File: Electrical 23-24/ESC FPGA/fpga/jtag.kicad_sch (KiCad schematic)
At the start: 0 parts

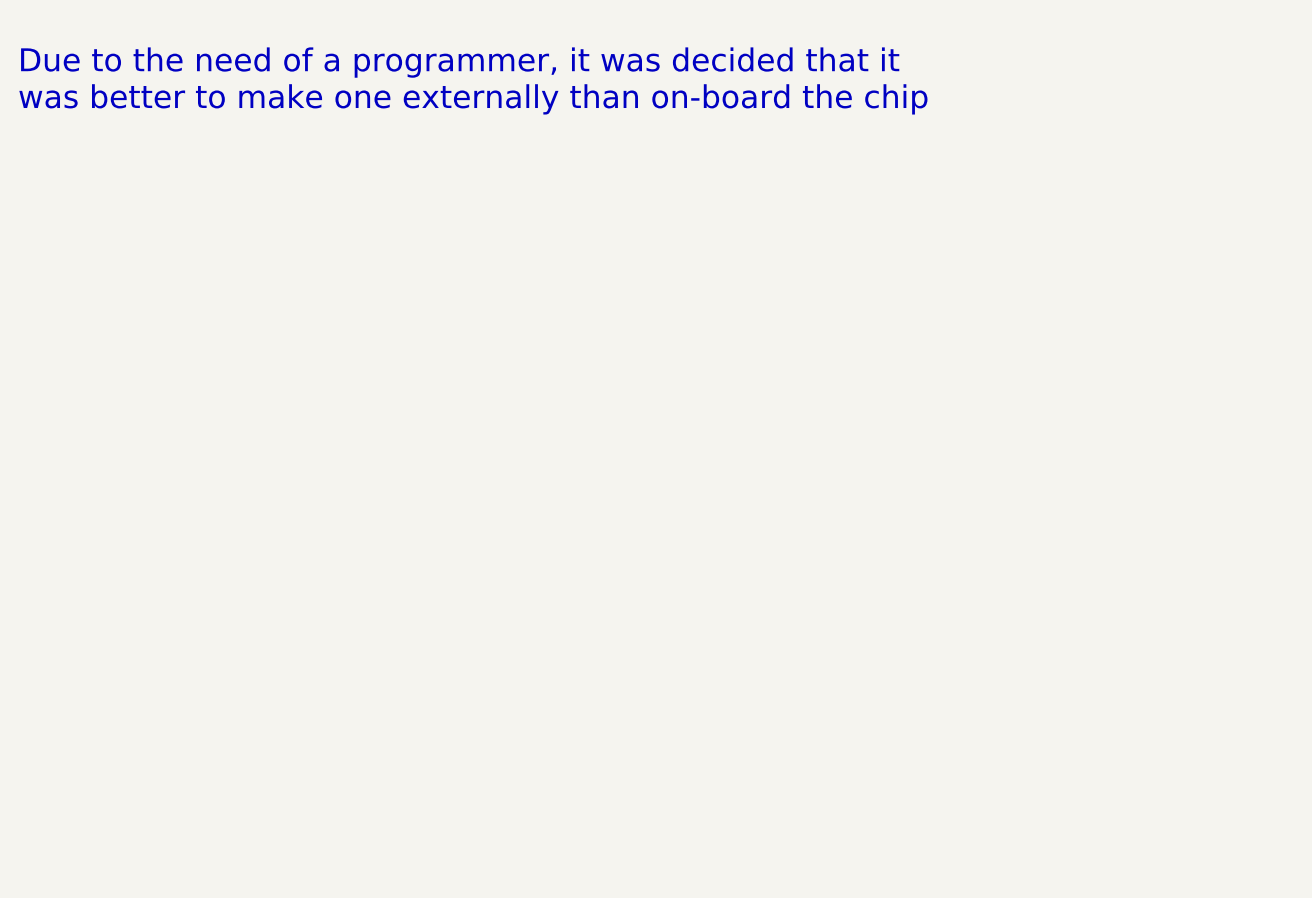
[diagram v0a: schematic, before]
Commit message: idk but something
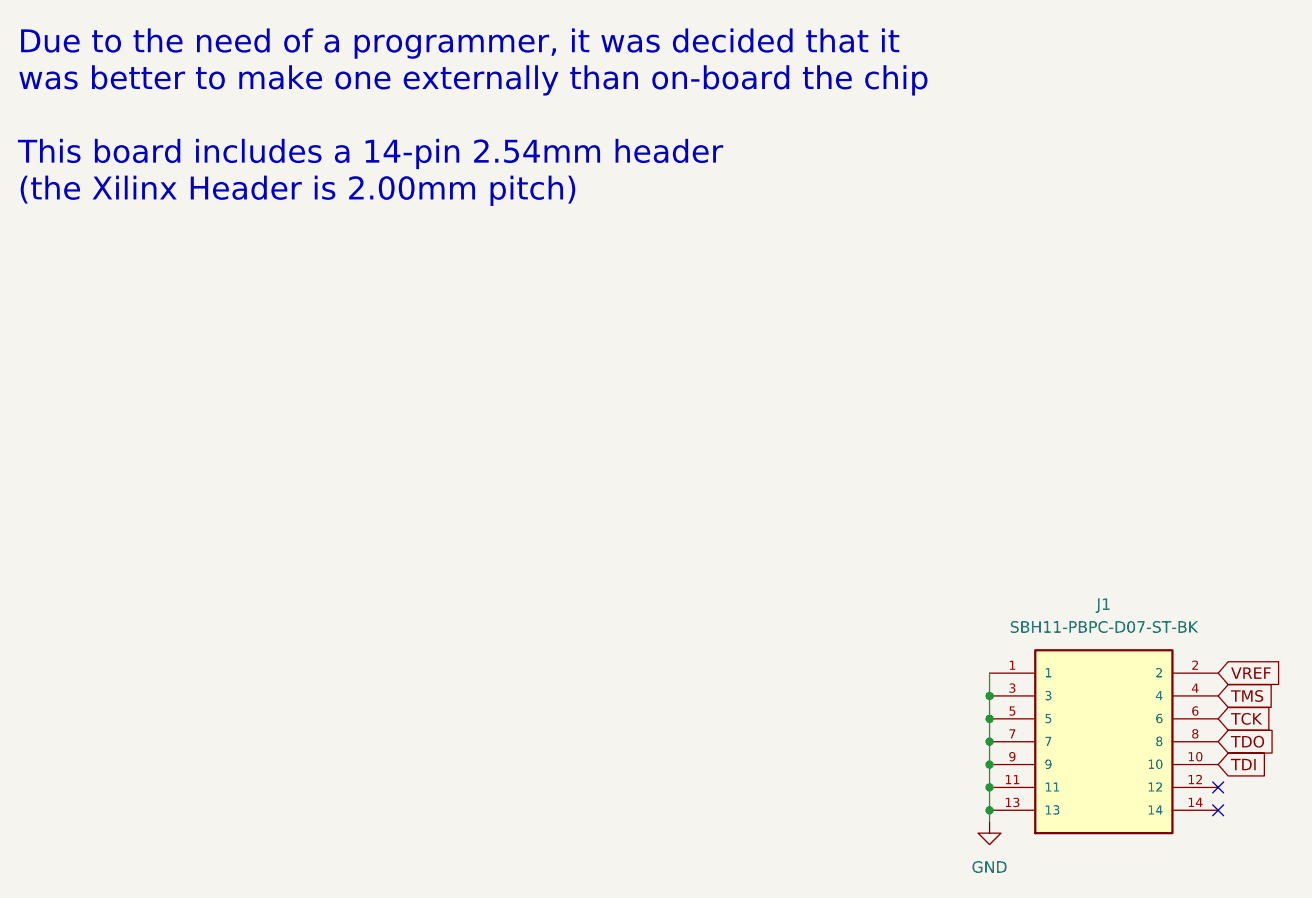
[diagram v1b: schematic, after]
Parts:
- added J1: SBH11-PBPC-D07-ST-BK, programmer:SULLINS_SBH11-PBPC-D07-ST-BK, symbol programmer:SBH11-PBPC-D07-ST-BK
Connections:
- new net GND: J1.1, J1.11, J1.13, J1.3, J1.5, J1.7, J1.9
- new net TCK: J1.6
- new net TDI: J1.10
- new net TDO: J1.8
- new net TMS: J1.4
- new net VREF: J1.2
- no-connect marks 0 -> 2
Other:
- note added: "Due to the need of a programmer, it was decided that it was better to make one externally than on-board the chip This board includes a 14-pin 2.54mm header (the Xilinx Header is 2.00mm pitch)"
- note removed: "Due to the need of a programmer, it was decided that it was better to make one externally than on-board the chip"
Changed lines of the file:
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@@
 (kicad_sch (version 20230121) (generator eeschema)
   (paper "A4")
-  (text "Due to the need of a programmer, it was decided that it\nwas better to make one externally than on-board the chip"
-    (at 19.05 26.67 0)
+  (junction (at 127 91.44) (diameter 0) (color 0 0 0 0)
+  )
+  (junction (at 127 96.52) (diameter 0) (color 0 0 0 0)
+  )
+  (junction (at 127 104.14) (diameter 0) (color 0 0 0 0)
+  )
+  (junction (at 127 99.06) (diameter 0) (color 0 0 0 0)
+  )
+  (junction (at 127 101.6) (diameter 0) (color 0 0 0 0)
+  )
+  (junction (at 127 93.98) (diameter 0) (color 0 0 0 0)
+  )
+  (no_connect (at 152.4 101.6))
+  (no_connect (at 152.4 104.14))
+  (wire (pts (xy 127 91.44) (xy 127 93.98))
+    (stroke (width 0) (type default))
+  )
+  (wire (pts (xy 127 96.52) (xy 127 99.06))
+    (stroke (width 0) (type default))
+  )
+  (wire (pts (xy 127 88.9) (xy 127 91.44))
+    (stroke (width 0) (type default))
+  )
+  (wire (pts (xy 127 101.6) (xy 127 104.14))
+    (stroke (width 0) (type default))
+  )
+  (wire (pts (xy 127 93.98) (xy 127 96.52))
+    (stroke (width 0) (type default))
+  )
+  (wire (pts (xy 127 104.14) (xy 127 105.41))
+    (stroke (width 0) (type default))
+  )
+  (wire (pts (xy 127 99.06) (xy 127 101.6))
+    (stroke (width 0) (type default))
+  )
+  (text "Due to the need of a programmer, it was decided that it\nwas better to make one externally than on-board the chip\n\nThis board includes a 14-pin 2.54mm header\n(the Xilinx Header is 2.00mm pitch)"
+    (at 19.05 36.83 0)
     (effects (font (size 2.54 2.54)) (justify left bottom))
   )
+  (global_label "TDO" (shape input) (at 152.4 96.52 0) (fields_autoplaced)
+    (effects (font (size 1.27 1.27)) (justify left))
+    (property "Intersheetrefs" "${INTERSHEET_REFS}" (at 158.9533 96.52 0)
+      (effects (font (size 1.27 1.27)) (justify left) hide)
+    )
+  )
+  (global_label "VREF" (shape input) (at 152.4 88.9 0) (fields_autoplaced)
+    (effects (font (size 1.27 1.27)) (justify left))
+    (property "Intersheetrefs" "${INTERSHEET_REFS}" (at 159.9814 88.9 0)
+      (effects (font (size 1.27 1.27)) (justify left) hide)
+    )
+  )
+  (global_label "TMS" (shape input) (at 152.4 91.44 0) (fields_autoplaced)
+    (effects (font (size 1.27 1.27)) (justify left))
+    (property "Intersheetrefs" "${INTERSHEET_REFS}" (at 159.0137 91.44 0)
+      (effects (font (size 1.27 1.27)) (justify left) hide)
+    )
+  )
+  (global_label "TCK" (shape input) (at 152.4 93.98 0) (fields_autoplaced)
+    (effects (font (size 1.27 1.27)) (justify left))
+    (property "Intersheetrefs" "${INTERSHEET_REFS}" (at 158.8928 93.98 0)
+      (effects (font (size 1.27 1.27)) (justify left) hide)
+    )
+  )
+  (global_label "TDI" (shape input) (at 152.4 99.06 0) (fields_autoplaced)
+    (effects (font (size 1.27 1.27)) (justify left))
+    (property "Intersheetrefs" "${INTERSHEET_REFS}" (at 158.2276 99.06 0)
+      (effects (font (size 1.27 1.27)) (justify left) hide)
+    )
+  )
+  (symbol (lib_id "programmer:SBH11-PBPC-D07-ST-BK") (at 139.7 96.52 0) (unit 1)
+    (in_bom yes) (on_board yes) (dnp no) (fields_autoplaced)
+    (property "Reference" "J1" (at 139.7 81.28 0)
+      (effects (font (size 1.27 1.27)))
+    )
+    (property "Value" "SBH11-PBPC-D07-ST-BK" (at 139.7 83.82 0)
+      (effects (font (size 1.27 1.27)))
+    )
+    (property "Footprint" "programmer:SULLINS_SBH11-PBPC-D07-ST-BK" (at 139.7 96.52 0)
+      (effects (font (size 1.27 1.27)) (justify bottom) hide)
+    )
+    (property "Datasheet" "" (at 139.7 96.52 0)
+      (effects (font (size 1.27 1.27)) hide)
+    )
+    (property "PARTREV" "J" (at 139.7 96.52 0)
+      (effects (font (size 1.27 1.27)) (justify bottom) hide)
+    )
+    (property "STANDARD" "Manufacturer Recommendation" (at 139.7 96.52 0)
+      (effects (font (size 1.27 1.27)) (justify bottom) hide)
+    )
+    (property "MANUFACTURER" "Sullins" (at 139.7 96.52 0)
+      (effects (font (size 1.27 1.27)) (justify bottom) hide)
+    )
+    (pin "1")
+    (pin "10")
+    (pin "11")
+    (pin "12")
+    (pin "13")
+    (pin "14")
+    (pin "2")
+    (pin "3")
+    (pin "4")
+    (pin "5")
+    (pin "6")
+    (pin "7")
+    (pin "8")
+    (pin "9")
+    (instances
+      (project "fpga"
+        (path "/5bf59577-a814-4364-8f7a-37815cfb5474/3d3d8e49-9c73-4011-93e8-c0355c1f458a"
+          (reference "J1") (unit 1)
+        )
+      )
+    )
+  )
+  (symbol (lib_id "power:GND") (at 127 105.41 0) (unit 1)
+    (in_bom yes) (on_board yes) (dnp no) (fields_autoplaced)
+    (property "Reference" "#PWR09" (at 127 111.76 0)
+      (effects (font (size 1.27 1.27)) hide)
+    )
+    (property "Value" "GND" (at 127 110.49 0)
+      (effects (font (size 1.27 1.27)))
+    )
+    (property "Footprint" "" (at 127 105.41 0)
+      (effects (font (size 1.27 1.27)) hide)
+    )
+    (property "Datasheet" "" (at 127 105.41 0)
+      (effects (font (size 1.27 1.27)) hide)
+    )
+    (pin "1")
+    (instances
+      (project "fpga"
+        (path "/5bf59577-a814-4364-8f7a-37815cfb5474/3d3d8e49-9c73-4011-93e8-c0355c1f458a"
+          (reference "#PWR09") (unit 1)
+        )
+      )
+    )
+  )
 )
